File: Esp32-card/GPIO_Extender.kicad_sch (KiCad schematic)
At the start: 3 parts, among them U1 74HC595, U2 74HC595, U4 74HC4051

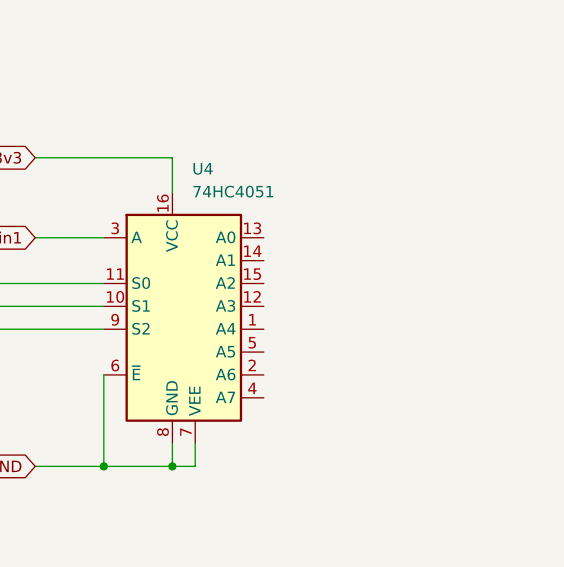
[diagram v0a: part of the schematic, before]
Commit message: Alimentation
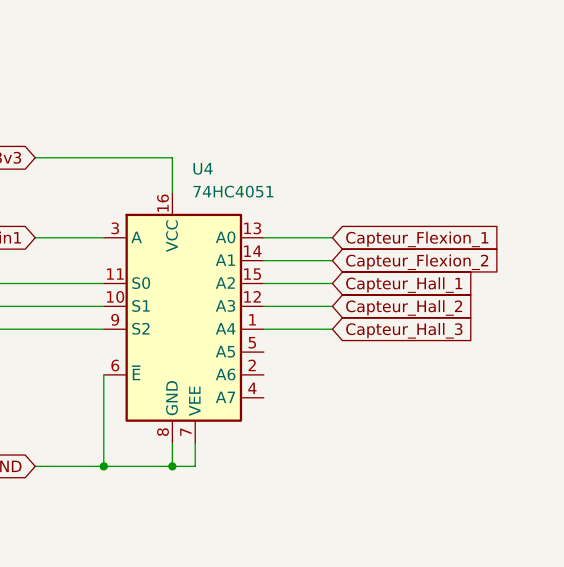
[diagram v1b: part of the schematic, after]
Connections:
- net Capteur_Hall_3: now reaches U4.1 (A4)
- net Capteur_Hall_2: now reaches U4.12 (A3)
- net Capteur_Flexion_1: now reaches U4.13 (A0)
- net Capteur_Flexion_2: now reaches U4.14 (A1)
- net Capteur_Hall_1: now reaches U4.15 (A2)
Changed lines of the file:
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@@
+	(wire
+		(pts
+			(xy 185.42 81.28) (xy 193.04 81.28)
+		)
+		(stroke
+			(width 0)
+			(type default)
+		)
+	)
 	(wire
 		(pts
@@
 	(wire
 		(pts
+			(xy 185.42 88.9) (xy 193.04 88.9)
+		)
+		(stroke
+			(width 0)
+			(type default)
+		)
+	)
+	(wire
+		(pts
 			(xy 115.57 57.15) (xy 128.27 57.15)
 		)
@@
 	(wire
 		(pts
+			(xy 185.42 86.36) (xy 193.04 86.36)
+		)
+		(stroke
+			(width 0)
+			(type default)
+		)
+	)
+	(wire
+		(pts
 			(xy 92.71 127) (xy 105.41 127)
 		)
@@
 	(wire
 		(pts
+			(xy 185.42 78.74) (xy 193.04 78.74)
+		)
+		(stroke
+			(width 0)
+			(type default)
+		)
+	)
+	(wire
+		(pts
 			(xy 115.57 99.06) (xy 137.16 99.06)
 		)
@@
 	(wire
 		(pts
+			(xy 185.42 83.82) (xy 193.04 83.82)
+		)
+		(stroke
+			(width 0)
+			(type default)
+		)
+	)
+	(wire
+		(pts
 			(xy 175.26 104.14) (xy 175.26 101.6)
 		)
@@
 		)
 	)
+	(global_label "Capteur_Hall_3"
+		(shape input)
+		(at 193.04 88.9 0)
+		(fields_autoplaced yes)
+		(effects
+			(font
+				(size 1.27 1.27)
+			)
+			(justify left)
+		)
+		(property "Intersheetrefs" "${INTERSHEET_REFS}"
+			(at 210.2973 88.9 0)
+			(effects
+				(font
+					(size 1.27 1.27)
+				)
+				(justify left)
+				(hide yes)
+			)
+		)
+	)
 	(global_label "Analog_Pin1"
 		(shape input)
@@
 		)
 	)
+	(global_label "Capteur_Hall_2"
+		(shape input)
+		(at 193.04 86.36 0)
+		(fields_autoplaced yes)
+		(effects
+			(font
+				(size 1.27 1.27)
+			)
+			(justify left)
+		)
+		(property "Intersheetrefs" "${INTERSHEET_REFS}"
+			(at 210.2973 86.36 0)
+			(effects
+				(font
+					(size 1.27 1.27)
+				)
+				(justify left)
+				(hide yes)
+			)
+		)
+	)
 	(global_label "3v3"
 		(shape input)
@@
 				(hide yes)
 			)
+		)
+	)
+	(global_label "Capteur_Flexion_1"
+		(shape input)
+		(at 193.04 78.74 0)
+		(fields_autoplaced yes)
+		(effects
+			(font
+				(size 1.27 1.27)
+			)
+			(justify left)
+		)
+		(property "Intersheetrefs" "${INTERSHEET_REFS}"
+			(at 213.2607 78.74 0)
+			(effects
+				(font
+					(size 1.27 1.27)
+				)
+				(justify left)
+				(hide yes)
+			)
+		)
+	)
+	(global_label "Capteur_Flexion_2"
+		(shape input)
+		(at 193.04 81.28 0)
+		(fields_autoplaced yes)
+		(effects
+			(font
+				(size 1.27 1.27)
+			)
+			(justify left)
+		)
+		(property "Intersheetrefs" "${INTERSHEET_REFS}"
+			(at 213.2607 81.28 0)
+			(effects
+				(font
+					(size 1.27 1.27)
+				)
+				(justify left)
+				(hide yes)
+			)
+		)
+	)
+	(global_label "Capteur_Hall_1"
+		(shape input)
+		(at 193.04 83.82 0)
+		(fields_autoplaced yes)
+		(effects
+			(font
+				(size 1.27 1.27)
+			)
+			(justify left)
+		)
+		(property "Intersheetrefs" "${INTERSHEET_REFS}"
+			(at 210.2973 83.82 0)
+			(effects
+				(font
+					(size 1.27 1.27)
+				)
+				(justify left)
+				(hide yes)
+			)

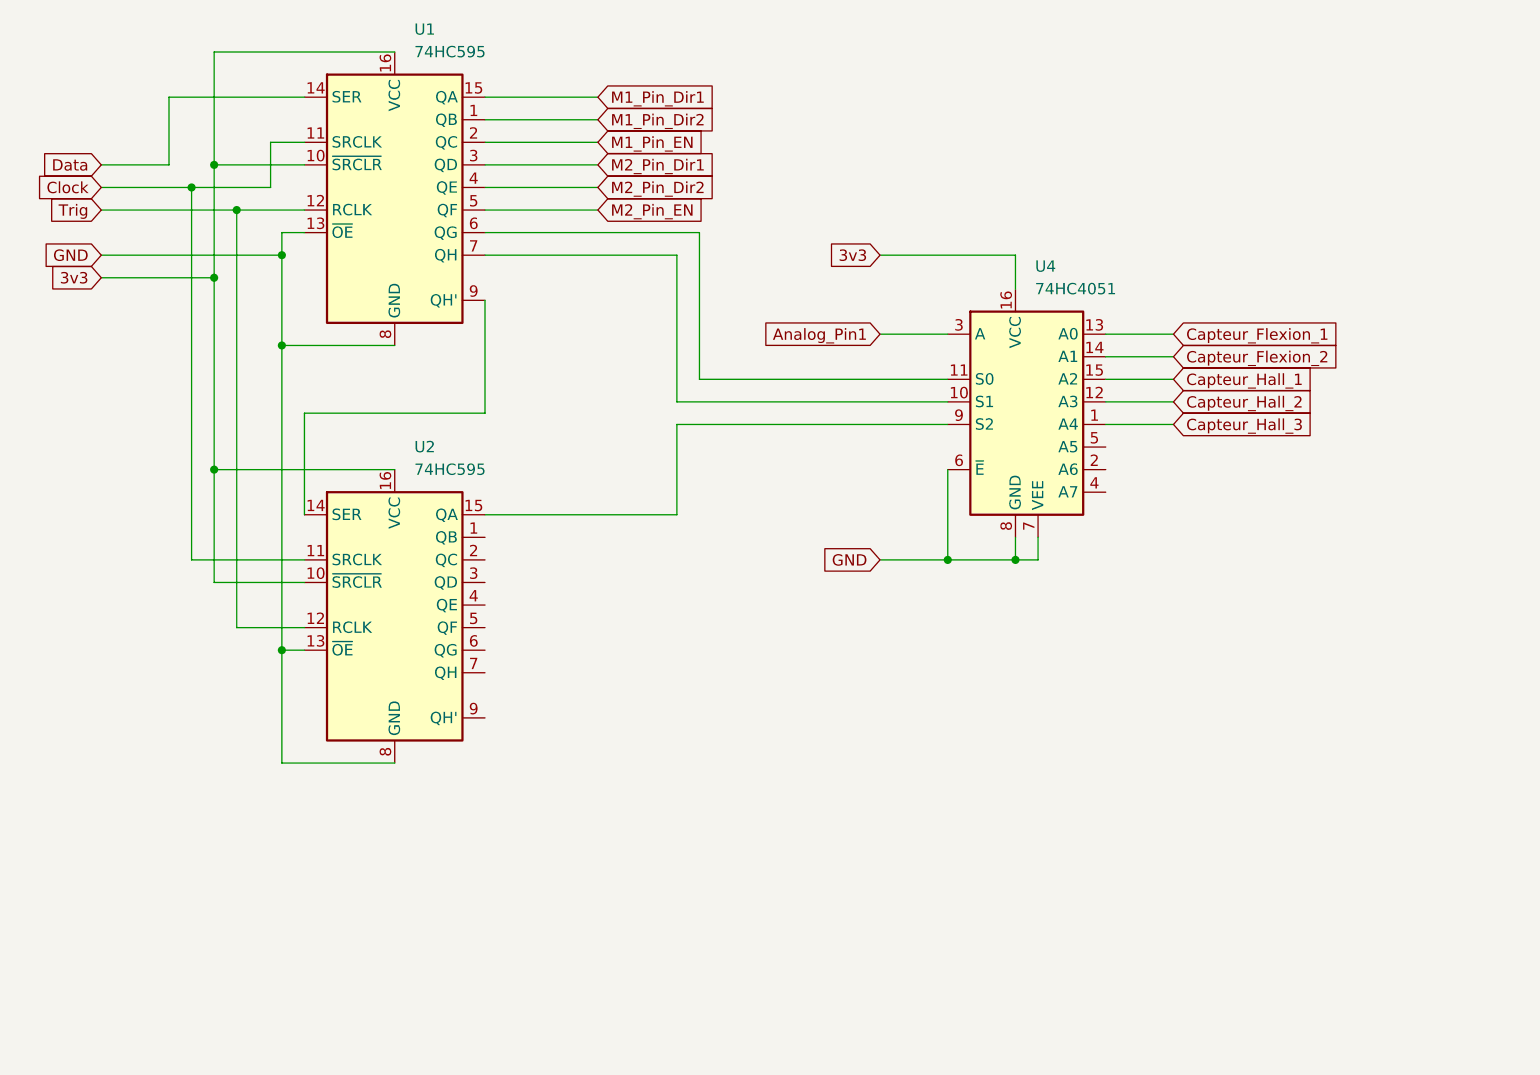
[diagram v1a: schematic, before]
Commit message: .
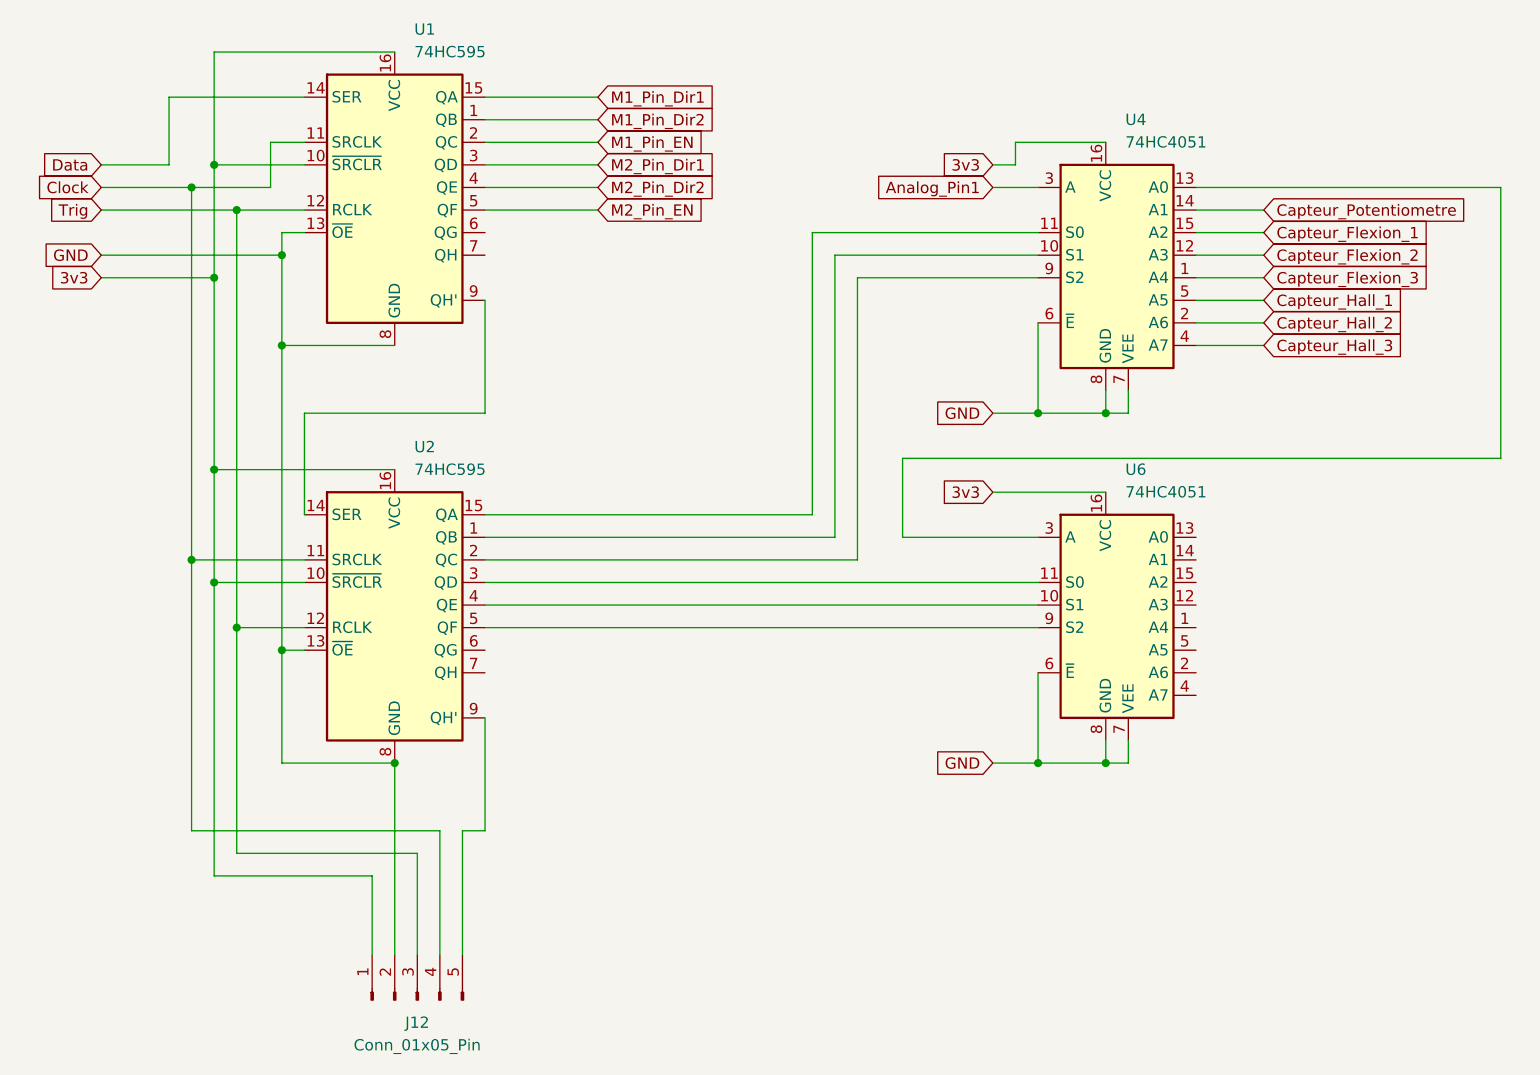
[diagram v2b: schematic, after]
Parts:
- added J12: Conn_01x05_Pin, symbol Connector:Conn_01x05_Pin
- added U6: 74HC4051, Package_DIP:DIP-16_W7.62mm, symbol 74xx:74HC4051
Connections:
- net 3v3: now also J12.1 (Pin_1), U6.16 (VCC)
- net Capteur_Flexion_1: now also U4.15 (A2); no longer U4.13 (A0)
- net Capteur_Flexion_2: now also U4.12 (A3); no longer U4.14 (A1)
- net Capteur_Hall_1: now also U4.5 (A5); no longer U4.15 (A2)
- net Capteur_Hall_2: now also U4.2 (A6); no longer U4.12 (A3)
- net Capteur_Hall_3: now also U4.4 (A7); no longer U4.1 (A4)
- net Clock: now also J12.4 (Pin_4)
- net GND: now also J12.2 (Pin_2), U6.6 (~{E}), U6.7 (VEE), U6.8 (GND)
- net Trig: now also J12.3 (Pin_3)
- net at U2.1 (QB): now also U4.10 (S1)
- net at U2.15 (QA): now also U4.11 (S0); no longer U4.9 (S2)
- net at U2.2 (QC): now also U4.9 (S2)
- net at U2.3 (QD): now also U6.11 (S0)
- net at U2.4 (QE): now also U6.10 (S1)
- net at U2.5 (QF): now also U6.9 (S2)
- net at U2.9 (QH'): now also J12.5 (Pin_5)
- net at U1.7 (QH): no longer U4.10 (S1)
- net at U1.6 (QG): no longer U4.11 (S0)
- new net: U4.13 (A0), U6.3 (A)
- new net Capteur_Flexion_3: U4.1 (A4)
- new net Capteur_Potentiometre: U4.14 (A1)
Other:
- moved on the sheet: U4
